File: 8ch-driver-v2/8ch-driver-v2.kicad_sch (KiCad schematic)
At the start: 36 parts, among them J1 Barrel_Jack, J2 Screw_Terminal_01x08, J3 Screw_Terminal_01x08, J4 Screw_Terminal_01x14, Q1 2N7002E, Q2 2N7002E, U1 DRV104PWP, U2 DRV104PWP

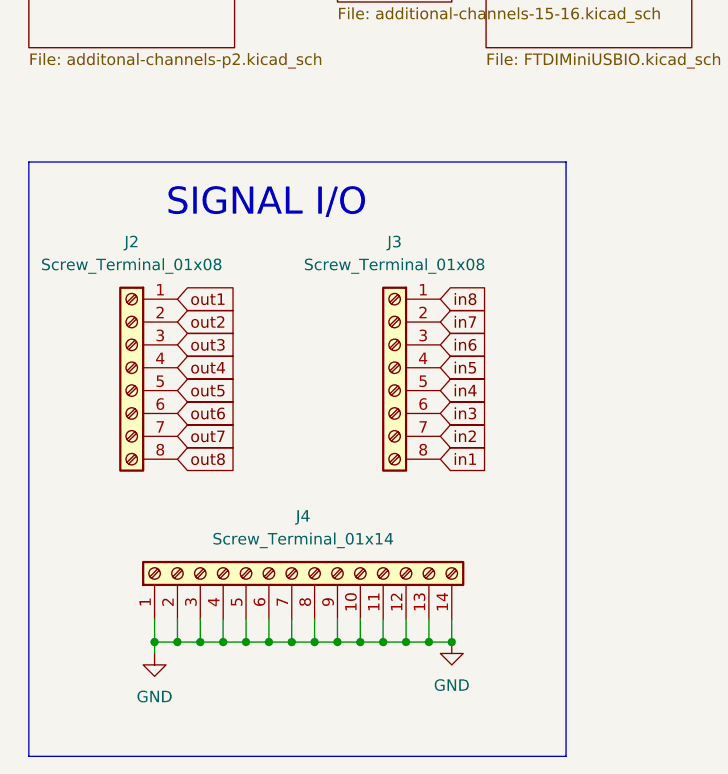
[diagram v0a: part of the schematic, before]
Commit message: progress
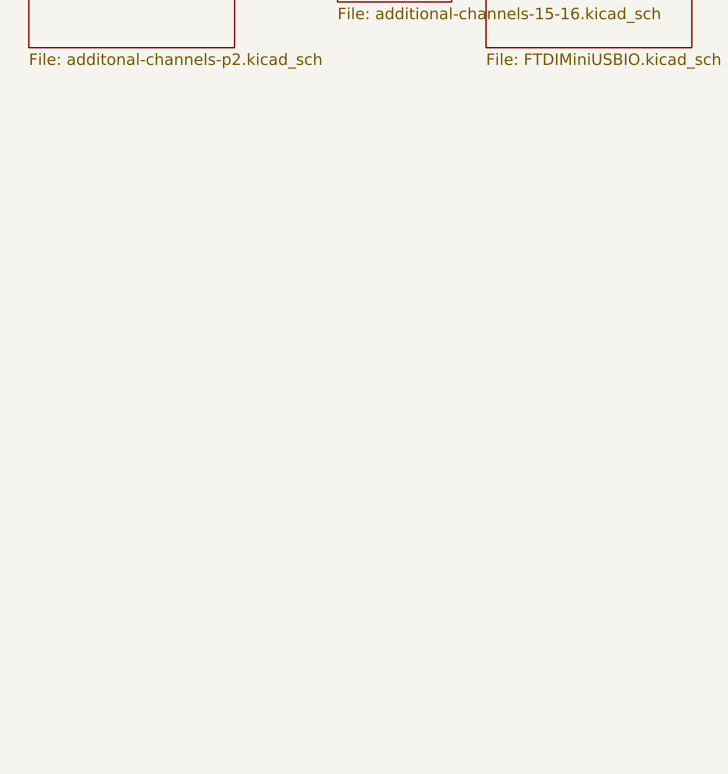
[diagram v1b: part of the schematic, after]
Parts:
- removed J2, J3: Screw_Terminal_01x08, TerminalBlock_Phoenix:TerminalBlock_Phoenix_PT-1,5-8-5.0-H_1x08_P5.00mm_Horizontal, symbol Connector:Screw_Terminal_01x08
- removed J4: Screw_Terminal_01x14, TerminalBlock_Phoenix:TerminalBlock_Phoenix_PT-1,5-14-5.0-H_1x14_P5.00mm_Horizontal, symbol Connector:Screw_Terminal_01x14
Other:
- note removed: "SIGNAL I/O"

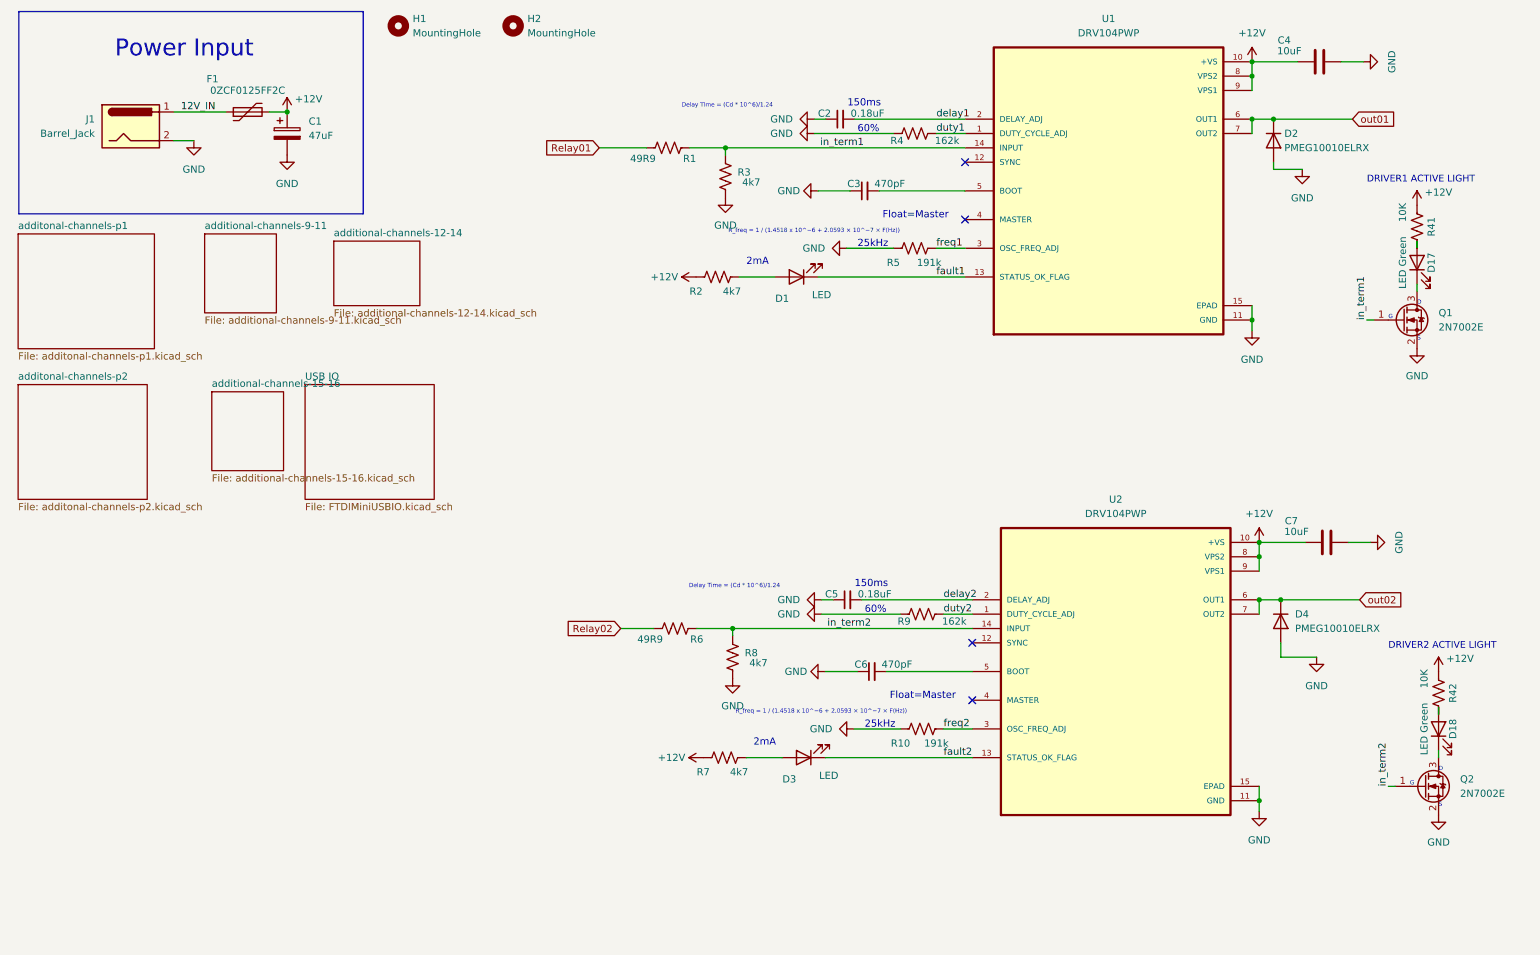
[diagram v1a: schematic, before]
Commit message: mucho mas progresso
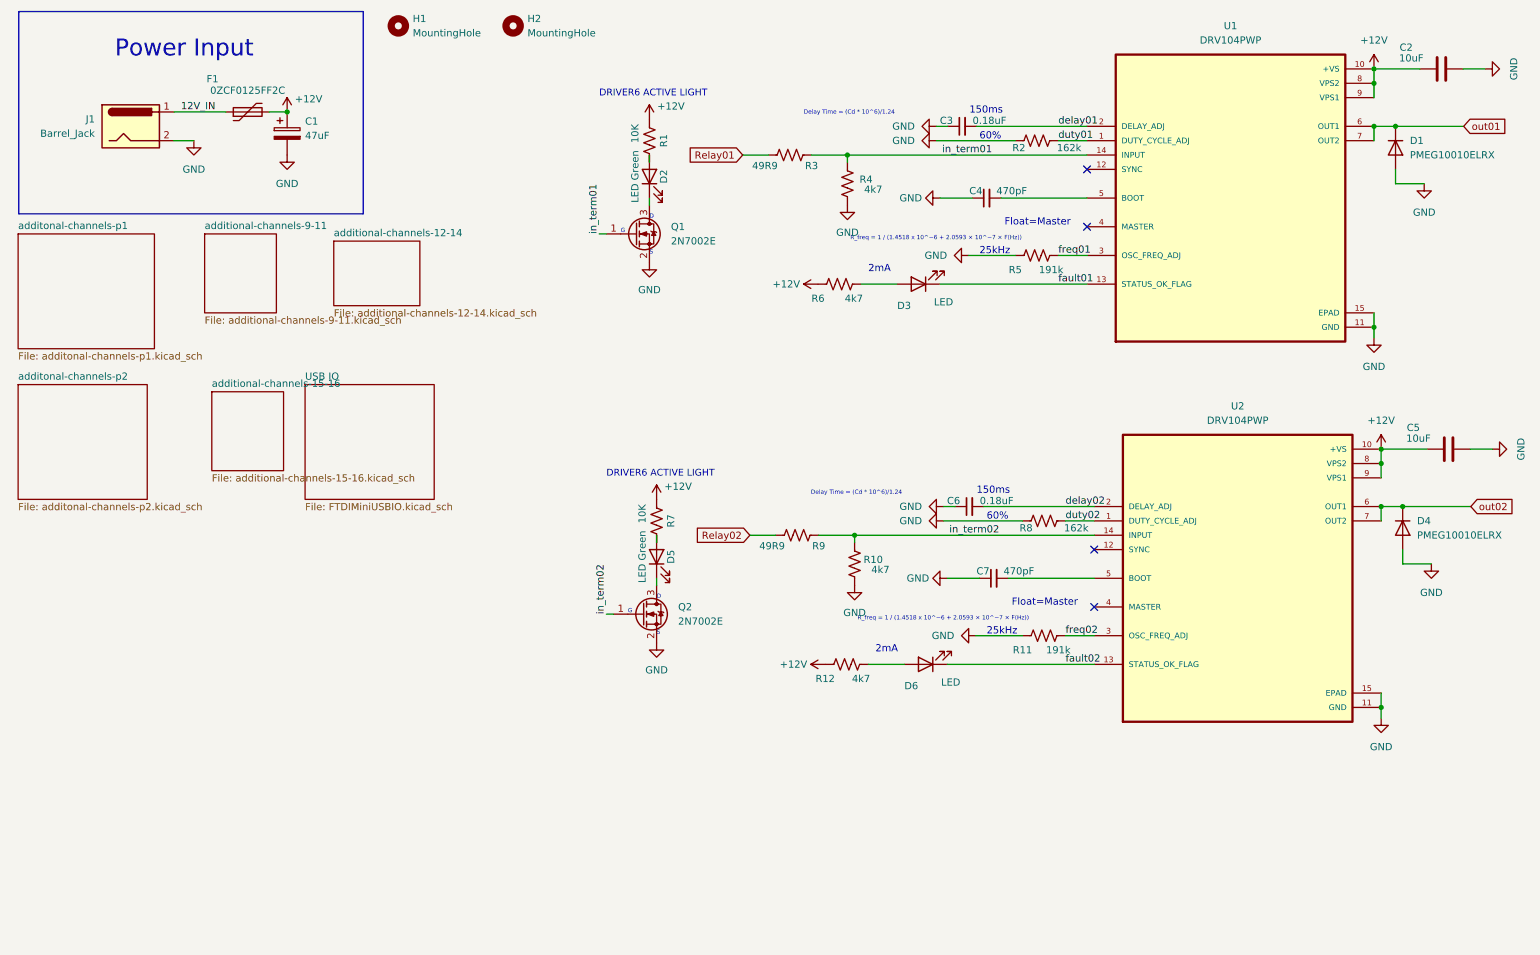
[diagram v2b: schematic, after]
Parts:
- removed C2, C5: 0.18uF, Capacitor_SMD:C_1206_3216Metric, symbol Device:C_Small
- removed C4, C7: 10uF, Capacitor_SMD:C_1210_3225Metric, symbol Device:C
- removed D1: LED, LED_SMD:LED_0805_2012Metric, symbol Device:LED
- removed D17, D18: LED Green, LED_SMD:LED_0805_2012Metric, symbol Device:LED
- removed D2: PMEG10010ELRX, Diode_SMD:Nexperia_CFP3_SOD-123W, symbol Device:D
- removed R41, R42: 10K, Resistor_SMD:R_1206_3216Metric, symbol Device:R_US
- added C2, C5: 10uF, Capacitor_SMD:C_1210_3225Metric, symbol Device:C
- added C4, C7: 470pF, Capacitor_SMD:C_1206_3216Metric, symbol Device:C_Small
- added D1: PMEG10010ELRX, Diode_SMD:Nexperia_CFP3_SOD-123W, symbol Device:D
- added D2, D5: LED Green, LED_SMD:LED_0805_2012Metric, symbol Device:LED
- added D6: LED, LED_SMD:LED_0805_2012Metric, symbol Device:LED
- added R11: 191k, Resistor_SMD:R_1206_3216Metric, symbol Device:R_US
- added R12: 4k7, Resistor_SMD:R_1206_3216Metric, symbol Device:R_US
- C3, C6: value 470pF -> 0.18uF; Mfg Kemet -> KYOCERA AVX; PartNum C0805C471K5RAC7800 -> 08053C184KAT2A
- R1: value 49R9 -> 10K; PartNum RC0805FR-0749R9L -> RC0805FR-07162KL
- R10: value 191k -> 4k7; PartNum RC0805FR-07191KL -> RC0805JR-074K7L
- R2, R8: value 4k7 -> 162k; PartNum RC0805JR-074K7L -> RC0805FR-07162KL
- R3: value 4k7 -> 49R9; PartNum RC0805JR-074K7L -> RC0805FR-0749R9L
- R4: value 162k -> 4k7; PartNum RC0805FR-07162KL -> RC0805JR-074K7L
- R6: value 49R9 -> 4k7; PartNum RC0805FR-0749R9L -> RC0805JR-074K7L
- R7: value 4k7 -> 10K; PartNum RC0805JR-074K7L -> RC0805FR-07162KL
- R9: value 162k -> 49R9; PartNum RC0805FR-07162KL -> RC0805FR-0749R9L
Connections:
- net +12V: now also R1.1, R6.1, C2.1, C5.1, R12.1; no longer R2.1
- net GND: now also R2.1, C2.2, C4.1, C5.2, C7.1, D1.2 (A), R11.1; no longer R3.1, R9.1
- net Relay01: now also R3.1; no longer R1.1
- net Relay02: now also R9.1; no longer R6.1
- net out01: now also D1.1 (K)
- net at U1.5 (BOOT): now also C4.2; no longer C3.2
- net at R7.2: now also D5.2 (A); no longer D3.2 (A)
- net at U2.5 (BOOT): now also C7.2; no longer C6.2
- net at Q2.3 (D): now also D5.1 (K)
- net duty01: now reaches R2.2
- net duty01: now also U1.1 (DUTY_CYCLE_ADJ)
- net at Q1.3 (D): now also D2.1 (K)
- net delay1 renamed delay01
- net delay01: now also C3.2
- net delay2 renamed delay02
- net delay02: now also C6.2
- net duty1 renamed in_term01
- net in_term01: now also Q1.1 (G), R3.2, U1.14 (INPUT); no longer U1.1 (DUTY_CYCLE_ADJ)
- net duty2 renamed duty02
- net duty02: now also R8.2; no longer R9.2
- net fault1 renamed fault01
- net fault01: now also D3.1 (K)
- net fault2 renamed fault02
- net fault02: now also D6.1 (K); no longer D3.1 (K)
- net freq1 renamed freq01
- net freq2 renamed freq02
- net freq02: now also R11.2; no longer R10.2
- removed net in_term1: Q1.1 (G), R1.2, R3.2, U1.14 (INPUT)
- net in_term2 renamed in_term02
- net in_term02: now also R10.2, R9.2; no longer R6.2, R8.2
- new net: D3.2 (A), R6.2
- new net: D2.2 (A), R1.2
- new net: D6.2 (A), R12.2
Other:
- note added: "DRIVER6 ACTIVE LIGHT"
- note removed: "DRIVER1 ACTIVE LIGHT"
- note removed: "DRIVER2 ACTIVE LIGHT"
